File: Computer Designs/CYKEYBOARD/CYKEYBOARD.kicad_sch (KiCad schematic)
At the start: 404 parts, among them J1 Conn_01x12, J2 Conn_01x03, J3 Conn_01x03, K0 RESET, K1 F1, K10 F10, K11 F11, K12 F12, K13 READY, K14 ~~,,,,,,`, K15 !,,,,,,1, K16 @,,,,,,2, K17 #,,,,,,3, K18 $,,,,,,4, K19 %,,,,,,5, K2 F2, K20 ^,,,,,,6, K21 &,,,,,,7, K22 *,,,,,,8, K23 (,,,,,,9, K24 ),,,,,,0, K25 _,,,,,,-, K26 +,,,,,,=, K27 BACKSPACE, K28 INS, K29 HOME, K3 F3, K30 !,,,,,,1, K31 SAVE,,,,,,LOAD, K32 Q, K33 W, K34 E, K35 R, K36 T, K37 Y, K38 U, K39 I, K4 F4, K40 O, K41 P, K42 {,,,,,,[, K43 },,,,,,], K44 |,,,,,,\, K45 DEL, K46 HOLD, K47 @,,,,,,2, K48 SHIFT,,,,,,LOCK, K49 A, K5 F5, K50 S, K51 D, K52 F, K53 G, K54 H, K55 J, K56 K, K57 L, K58 :,,,,,,;, K59 ",,,,,,', K6 F6, K60 ENTER, K61 SHIFT, K62 Z, K63 X, K64 C, K65 V, K66 B, K67 N, K68 M, K69 <,,,,,,,, K7 F7, K70 >,,,,,,., K71 ?,,,,,,/, K72 SHIFT, K73 ^, K74 CTRL, K75 CYKA,,,,,,TECH, K76 ALT, K77 Blank, K78 ALT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

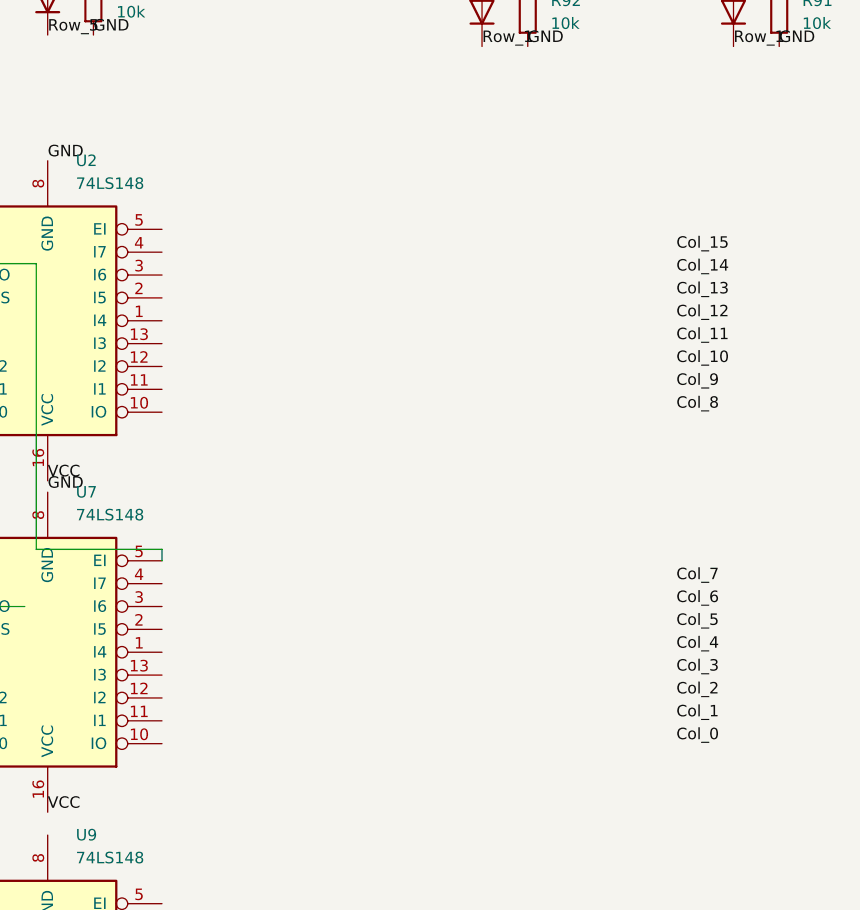
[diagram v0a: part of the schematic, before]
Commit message: Continued
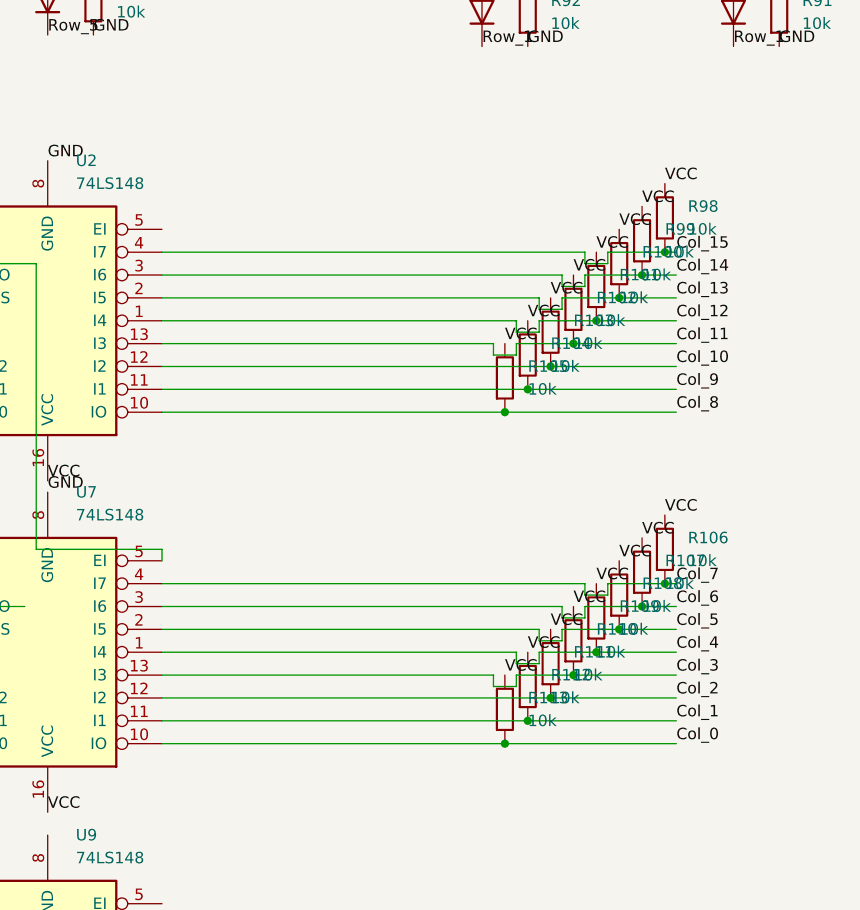
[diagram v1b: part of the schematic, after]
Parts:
- added R100, R101, R102, R103, R104, R105, R106, R107, R108, R109, R110, R111, R112, R113, R98, R99: 10k, Resistor_THT:R_Axial_DIN0207_L6.3mm_D2.5mm_P10.16mm_Horizontal, symbol PCM_SL_Resistors:10k
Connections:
- net Col_0: now also U7.10 (IO), R113.1
- net Col_1: now also U7.11 (I1), R112.1
- net Col_10: now also U2.12 (I2), R103.1
- net Col_11: now also U2.13 (I3), R102.1
- net Col_12: now also U2.1 (I4), R101.1
- net Col_13: now also U2.2 (I5), R100.1
- net Col_14: now also U2.3 (I6), R99.1
- net Col_15: now also U2.4 (I7), R98.1
- net Col_2: now also U7.12 (I2), R111.1
- net Col_3: now also U7.13 (I3), R110.1
- net Col_4: now also U7.1 (I4), R109.1
- net Col_5: now also U7.2 (I5), R108.1
- net Col_6: now also U7.3 (I6), R107.1
- net Col_7: now also U7.4 (I7), R106.1
- net Col_8: now also U2.10 (IO), R105.1
- net Col_9: now also U2.11 (I1), R104.1
- net VCC: now also R100.2, R101.2, R102.2, R103.2, R104.2, R105.2, R106.2, R107.2, R108.2, R109.2, R110.2, R111.2, R112.2, R113.2, R98.2, R99.2
